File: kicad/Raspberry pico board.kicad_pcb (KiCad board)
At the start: 2 copper layers, 24.8 x 96.5 mm, 11 parts, among them J1 Conn_01x20_Socket, J2 Conn_01x20_Socket, U2 MCP3301, U3 OPA340P, U4 C12666MA, U5 SN74AHCT125N, U6 SN74AHCT125N, U7 MCP1541-I/TO

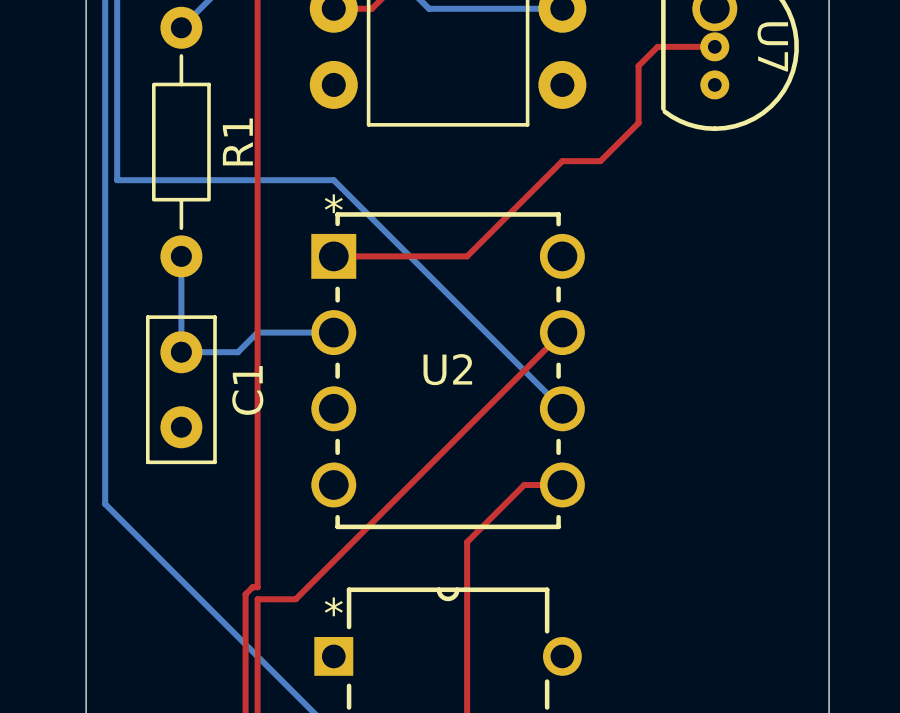
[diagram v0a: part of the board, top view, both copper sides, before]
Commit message: Schematic V2.0 finally made it work :)
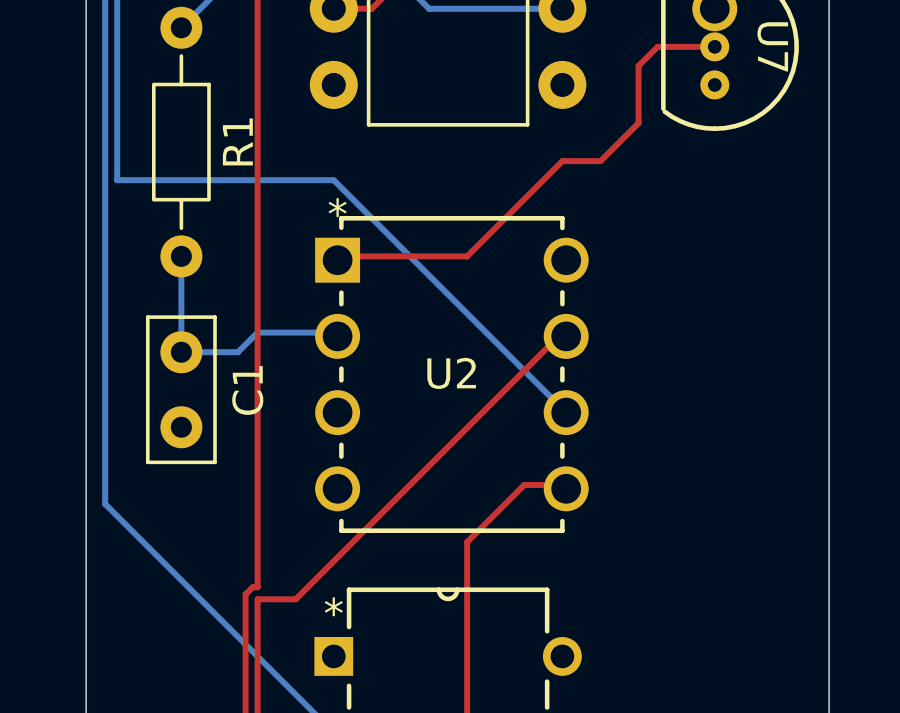
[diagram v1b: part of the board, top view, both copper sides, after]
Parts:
- moved U2 0.18 mm to (137.9, 87.1)
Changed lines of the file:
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@@
 	(footprint "Library JII FP:MCP3301_BI_P"
 		(layer "F.Cu")
-		(at 137.795 86.995)
+		(at 137.922 87.122)
 		(tags "MCP3301-BI/P ")
 		(property "Reference" "U2"
@@
 	)
 	(segment
-		(start 147.955 80.645)
-		(end 148.59 80.01)
-		(width 0.2)
-		(layer "F.Cu")
-		(net "Net-(U2-Vref)")
-	)
-	(segment
-		(start 142.24 86.995)
-		(end 145.415 83.82)
-		(width 0.2)
-		(layer "F.Cu")
-		(net "Net-(U2-Vref)")
-	)
-	(segment
-		(start 147.955 82.55)
-		(end 147.955 80.645)
-		(width 0.2)
-		(layer "F.Cu")
-		(net "Net-(U2-Vref)")
-	)
-	(segment
-		(start 137.795 86.995)
-		(end 142.24 86.995)
-		(width 0.2)
-		(layer "F.Cu")
-		(net "Net-(U2-Vref)")
-	)
-	(segment
-		(start 146.685 83.82)
-		(end 147.955 82.55)
-		(width 0.2)
-		(layer "F.Cu")
-		(net "Net-(U2-Vref)")
-	)
-	(segment
-		(start 145.415 83.82)
-		(end 146.685 83.82)
-		(width 0.2)
-		(layer "F.Cu")
-		(net "Net-(U2-Vref)")
-	)
-	(segment
-		(start 148.59 80.01)
-		(end 150.495 80.01)
-		(width 0.2)
-		(layer "F.Cu")
-		(net "Net-(U2-Vref)")
-	)
-	(segment
-		(start 136.525 105.41)
-		(end 135.255 104.14)
-		(width 0.2)
-		(layer "F.Cu")
-		(net "Net-(U2-CLK)")
-	)
-	(segment
-		(start 137.795 105.41)
-		(end 136.525 105.41)
-		(width 0.2)
-		(layer "F.Cu")
-		(net "Net-(U2-CLK)")
-	)
-	(segment
-		(start 135.255 104.14)
-		(end 135.255 98.425)
-		(width 0.2)
-		(layer "F.Cu")
-		(net "Net-(U2-CLK)")
-	)
-	(segment
-		(start 135.255 98.425)
-		(end 136.525 98.425)
-		(width 0.2)
-		(layer "F.Cu")
-		(net "Net-(U2-CLK)")
-	)
-	(segment
-		(start 136.525 98.425)
-		(end 145.415 89.535)
-		(width 0.2)
-		(layer "F.Cu")
-		(net "Net-(U2-CLK)")
-	)
-	(segment
-		(start 132.715 86.995)
-		(end 132.715 90.19)
-		(width 0.2)
-		(layer "B.Cu")
-		(net "Net-(U2-IN+)")
-	)
-	(segment
-		(start 135.255 89.535)
-		(end 137.795 89.535)
-		(width 0.2)
-		(layer "B.Cu")
-		(net "Net-(U2-IN+)")
-	)
-	(segment
-		(start 132.715 90.19)
-		(end 134.6 90.19)
-		(width 0.2)
-		(layer "B.Cu")
-		(net "Net-(U2-IN+)")
-	)
-	(segment
-		(start 134.6 90.19)
-		(end 135.255 89.535)
-		(width 0.2)
-		(layer "B.Cu")
-		(net "Net-(U2-IN+)")
-	)
-	(segment
-		(start 142.24 108.585)
-		(end 142.24 96.52)
-		(width 0.2)
-		(layer "F.Cu")
-		(net "Net-(U2-~{CS}{slash}SHDN)")
-	)
-	(segment
-		(start 137.795 113.03)
-		(end 142.24 108.585)
-		(width 0.2)
-		(layer "F.Cu")
-		(net "Net-(U2-~{CS}{slash}SHDN)")
-	)
-	(segment
-		(start 142.24 96.52)
-		(end 144.145 94.615)
-		(width 0.2)
-		(layer "F.Cu")
-		(net "Net-(U2-~{CS}{slash}SHDN)")
-	)
-	(segment
-		(start 144.145 94.615)
-		(end 145.415 94.615)
-		(width 0.2)
-		(layer "F.Cu")
-		(net "Net-(U2-~{CS}{slash}SHDN)")
-	)
-	(segment
 		(start 139.065 78.74)
 		(end 137.795 78.74)
@@
 	)
 	(segment
+		(start 132.715 86.995)
+		(end 132.715 90.19)
+		(width 0.2)
+		(layer "B.Cu")
+		(net "Net-(U2-IN+)")
+	)
+	(segment
+		(start 135.255 89.535)
+		(end 137.795 89.535)
+		(width 0.2)
+		(layer "B.Cu")
+		(net "Net-(U2-IN+)")
+	)
+	(segment
+		(start 132.715 90.19)
+		(end 134.6 90.19)
+		(width 0.2)
+		(layer "B.Cu")
+		(net "Net-(U2-IN+)")
+	)
+	(segment
+		(start 134.6 90.19)
+		(end 135.255 89.535)
+		(width 0.2)
+		(layer "B.Cu")
+		(net "Net-(U2-IN+)")
+	)
+	(segment
+		(start 130.175 95.25)
+		(end 137.795 102.87)
+		(width 0.2)
+		(layer "B.Cu")
+		(net "Net-(J2-Pin_17)")
+	)
+	(segment
+		(start 133.35 67.31)
+		(end 130.175 70.485)
+		(width 0.2)
+		(layer "B.Cu")
+		(net "Net-(J2-Pin_17)")
+	)
+	(segment
+		(start 130.175 70.485)
+		(end 130.175 95.25)
+		(width 0.2)
+		(layer "B.Cu")
+		(net "Net-(J2-Pin_17)")
+	)
+	(segment
+		(start 136.525 105.41)
+		(end 135.255 104.14)
+		(width 0.2)
+		(layer "F.Cu")
+		(net "Net-(U2-CLK)")
+	)
+	(segment
+		(start 137.795 105.41)
+		(end 136.525 105.41)
+		(width 0.2)
+		(layer "F.Cu")
+		(net "Net-(U2-CLK)")
+	)
+	(segment
+		(start 135.255 104.14)
+		(end 135.255 98.425)
+		(width 0.2)
+		(layer "F.Cu")
+		(net "Net-(U2-CLK)")
+	)
+	(segment
+		(start 135.255 98.425)
+		(end 136.525 98.425)
+		(width 0.2)
+		(layer "F.Cu")
+		(net "Net-(U2-CLK)")
+	)
+	(segment
+		(start 136.525 98.425)
+		(end 145.415 89.535)
+		(width 0.2)
+		(layer "F.Cu")
+		(net "Net-(U2-CLK)")
+	)
+	(segment
 		(start 134.855 104.305685)
 		(end 134.855 98.259315)
@@
 	)
 	(segment
+		(start 142.24 108.585)
+		(end 142.24 96.52)
+		(width 0.2)
+		(layer "F.Cu")
+		(net "Net-(U2-~{CS}{slash}SHDN)")
+	)
+	(segment
+		(start 137.795 113.03)
+		(end 142.24 108.585)
+		(width 0.2)
+		(layer "F.Cu")
+		(net "Net-(U2-~{CS}{slash}SHDN)")
+	)
+	(segment
+		(start 142.24 96.52)
+		(end 144.145 94.615)
+		(width 0.2)
+		(layer "F.Cu")
+		(net "Net-(U2-~{CS}{slash}SHDN)")
+	)
+	(segment
+		(start 144.145 94.615)
+		(end 145.415 94.615)
+		(width 0.2)
+		(layer "F.Cu")
+		(net "Net-(U2-~{CS}{slash}SHDN)")
+	)
+	(segment
+		(start 147.955 80.645)
+		(end 148.59 80.01)
+		(width 0.2)
+		(layer "F.Cu")
+		(net "Net-(U2-Vref)")
+	)
+	(segment
+		(start 142.24 86.995)
+		(end 145.415 83.82)
+		(width 0.2)
+		(layer "F.Cu")
+		(net "Net-(U2-Vref)")
+	)
+	(segment
+		(start 147.955 82.55)
+		(end 147.955 80.645)
+		(width 0.2)
+		(layer "F.Cu")
+		(net "Net-(U2-Vref)")
+	)
+	(segment
+		(start 137.795 86.995)
+		(end 142.24 86.995)
+		(width 0.2)
+		(layer "F.Cu")
+		(net "Net-(U2-Vref)")
+	)
+	(segment
+		(start 146.685 83.82)
+		(end 147.955 82.55)
+		(width 0.2)
+		(layer "F.Cu")
+		(net "Net-(U2-Vref)")
+	)
+	(segment
+		(start 145.415 83.82)
+		(end 146.685 83.82)
+		(width 0.2)
+		(layer "F.Cu")
+		(net "Net-(U2-Vref)")
+	)
+	(segment
+		(start 148.59 80.01)
+		(end 150.495 80.01)
+		(width 0.2)
+		(layer "F.Cu")
+		(net "Net-(U2-Vref)")
+	)
+	(segment
 		(start 130.575 77.705)
 		(end 133.35 74.93)
@@
 	)
 	(segment
-		(start 130.175 95.25)
-		(end 137.795 102.87)
-		(width 0.2)
-		(layer "B.Cu")
-		(net "Net-(J2-Pin_17)")
-	)
-	(segment
-		(start 133.35 67.31)
-		(end 130.175 70.485)
-		(width 0.2)
-		(layer "B.Cu")
-		(net "Net-(J2-Pin_17)")
-	)
-	(segment
-		(start 130.175 70.485)
-		(end 130.175 95.25)
-		(width 0.2)
-		(layer "B.Cu")
-		(net "Net-(J2-Pin_17)")
-	)
-	(segment
 		(start 135.89 76.2)
 		(end 132.715 79.375)
@@
 	)
 	(segment
-		(start 133.367 36.857)
-		(end 133.394 36.83)
-		(width 0.2)
-		(layer "F.Cu")
-		(net "unconnected-(J2-Pin_5-Pad5)")
-	)
-	(segment
 		(start 133.367 34.317)
 		(end 133.361911 34.311911)
@@
 		(net "unconnected-(J2-Pin_4-Pad4)")
 	)
+	(segment
+		(start 133.367 36.857)
+		(end 133.394 36.83)
+		(width 0.2)
+		(layer "F.Cu")
+		(net "unconnected-(J2-Pin_5-Pad5)")
+	)
 	(zone
